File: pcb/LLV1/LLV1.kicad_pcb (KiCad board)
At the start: 2 copper layers, 4 parts, among them J2 Conn_01x02, SW1 SW_Push, U1 XIAO-nRF52840-SMD, U2 MAX30102

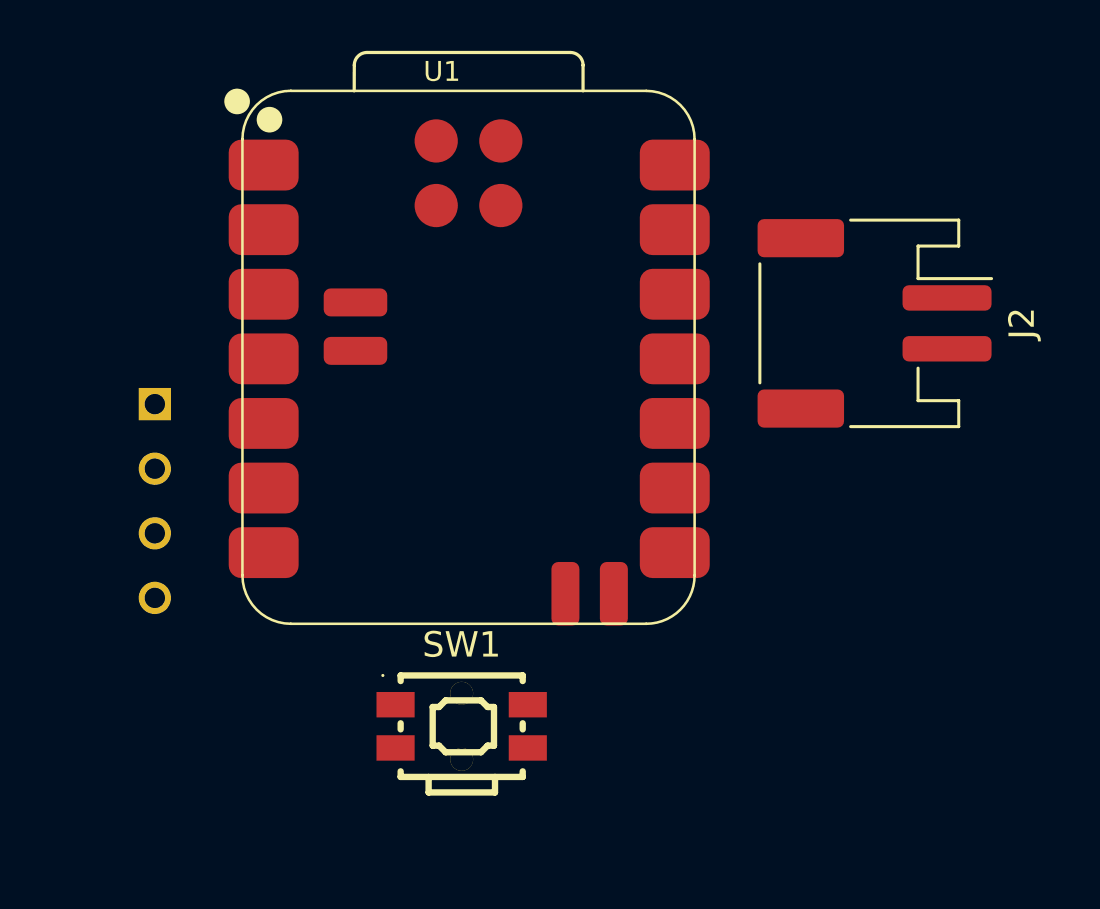
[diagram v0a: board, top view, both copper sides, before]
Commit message: Sync repo with latest code
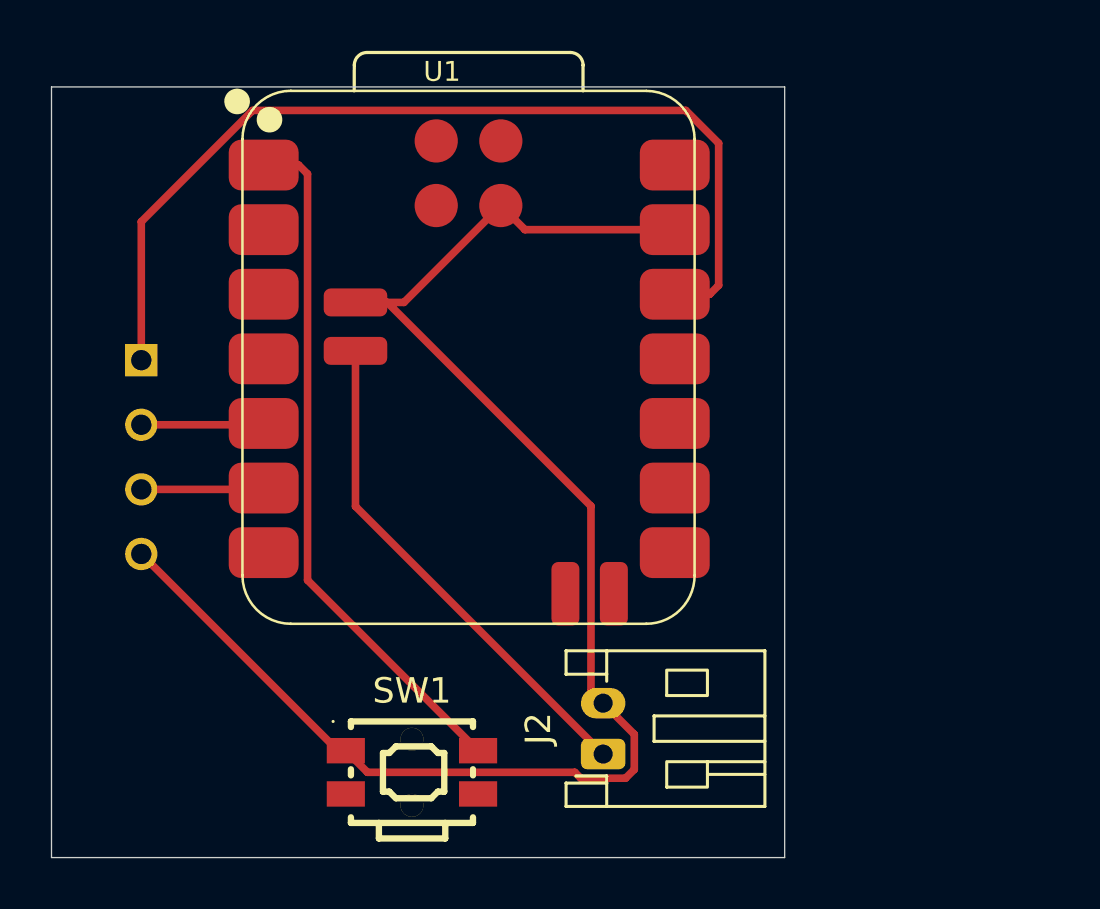
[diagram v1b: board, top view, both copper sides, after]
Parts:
- J2: footprint Connector_JST:JST_PH_S2B-PH-SM4-TB_1x02-1MP_P2.00mm_Horizontal -> Connector_JST:JST_PH_S2B-PH-K_1x02_P2.00mm_Horizontal
- moved J2 20.0 mm to (145.9, 149.7), turned to 90 degrees
- moved SW1 2.66 mm to (138.4, 150.4)
- moved U2 1.81 mm to (132.8, 138.0)
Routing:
- net GND: track 0.00 -> 61.3 mm
- net +3V3: track 0.00 -> 38.0 mm
- net Net-(U1-D0): track 0.00 -> 27.3 mm
- net Net-(J2-Pin_1): track 0.00 -> 19.9 mm
- net Net-(U1-D5): track 0.00 -> 4.83 mm
- net Net-(U1-D4): track 0.00 -> 4.83 mm
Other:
- board outline added: 28.8 x 30.3 mm
